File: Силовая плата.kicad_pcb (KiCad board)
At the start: 6 copper layers, 65.7 x 72.2 mm, 57 parts, among them J3 Conn_01x01, J4 Conn_01x01, J5 Conn_01x01, J6 Conn_02x04_Odd_Even, Q1 BSP89, Q2 BSP89, Q3 BSP89, Q4 BSP89, Q5 BSP89, Q6 BSP89, U1 LMV7239M5, U6 AD8210

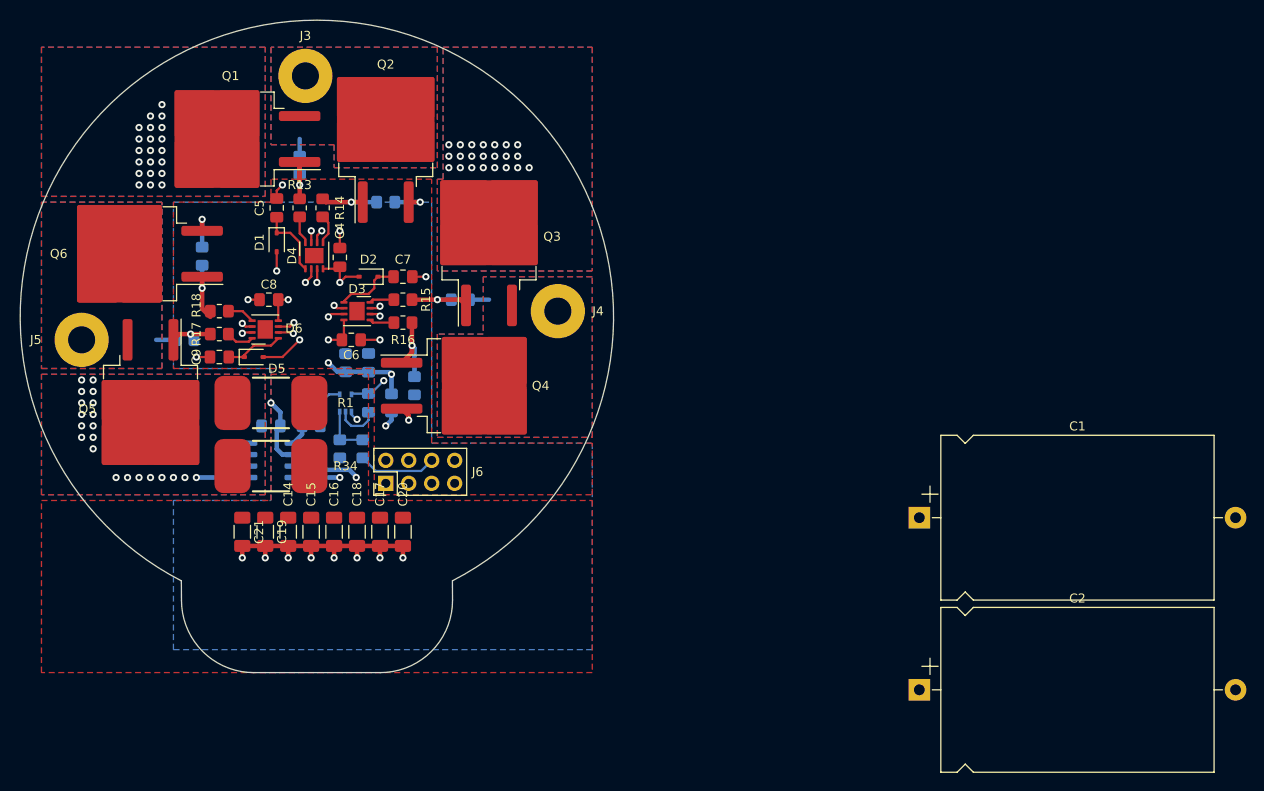
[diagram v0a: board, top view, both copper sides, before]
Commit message: Стартовая версия
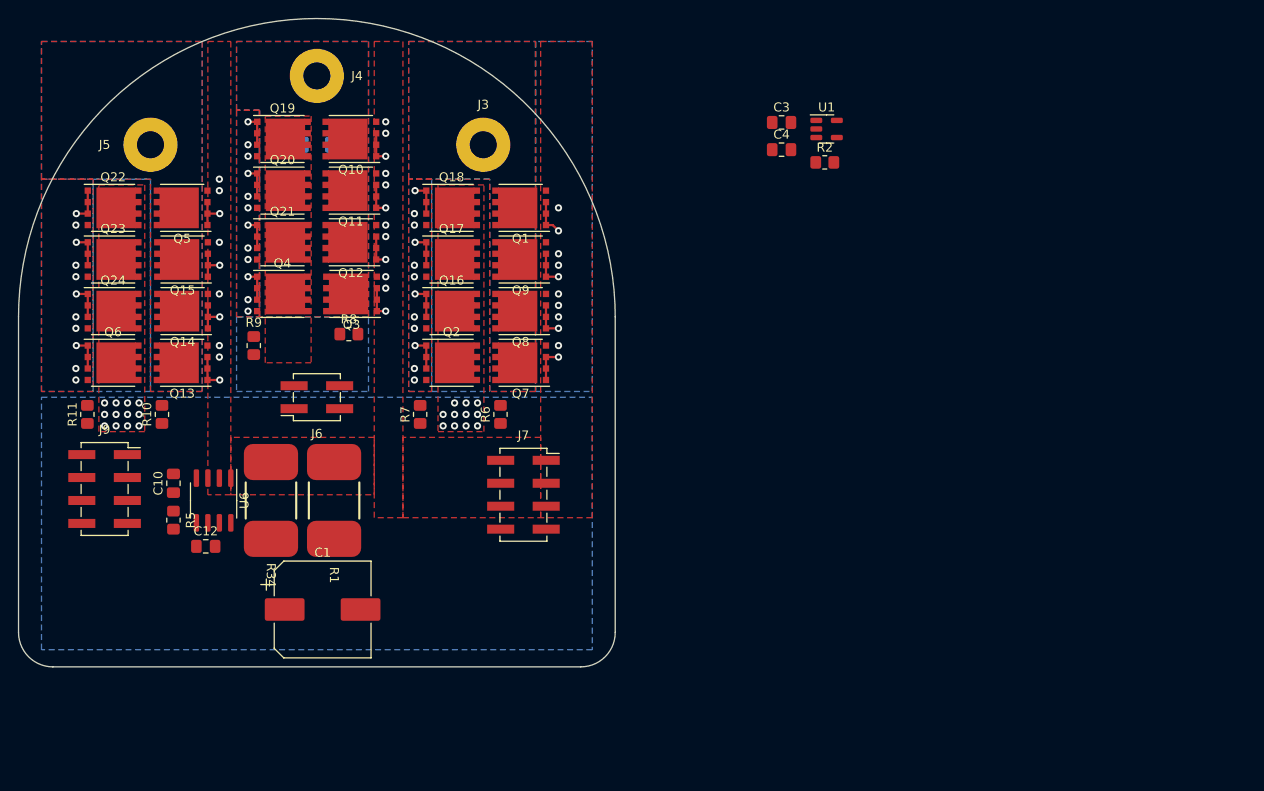
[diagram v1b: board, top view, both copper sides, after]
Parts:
- removed C11: 56p, Capacitor_SMD:C_0805_2012Metric_Pad1.18x1.45mm_HandSolder
- removed C14, C15, C16, C17, C18, C19, C20, C21: 4.7u, Capacitor_SMD:C_1206_3216Metric_Pad1.33x1.80mm_HandSolder
- removed C2: 1400m, Capacitor_THT:CP_Axial_L30.0mm_D18.0mm_P35.00mm_Horizontal
- removed C5, C7, C9: BS, Capacitor_SMD:C_0805_2012Metric_Pad1.18x1.45mm_HandSolder
- removed C6, C8: 10u, Capacitor_SMD:C_0805_2012Metric_Pad1.18x1.45mm_HandSolder
- removed D1, D2, D5: D_Small, Diode_SMD:D_SOD-323
- removed D3, D4, D6: ADP3110A, Package_DFN_QFN:DFN-8-1EP_3x3mm_P0.65mm_EP1.7x2.05mm
- removed R13, R14, R15, R16, R17, R18: 2.7, Resistor_SMD:R_0805_2012Metric_Pad1.20x1.40mm_HandSolder
- removed R21: 10k, Resistor_SMD:R_0805_2012Metric_Pad1.20x1.40mm_HandSolder
- removed R3, R4: 120, Resistor_SMD:R_0805_2012Metric_Pad1.20x1.40mm_HandSolder
- added J7: A_CTRL, Connector_PinSocket_2.54mm:PinSocket_2x04_P2.54mm_Vertical_SMD, F.Cu at (106.0, 114.3)
- added J9: C_CTRL, Connector_PinSocket_2.54mm:PinSocket_2x04_P2.54mm_Vertical_SMD, F.Cu at (59.7, 113.7)
- added Q10: BSP89, Package_SON:VSONP-8-1EP_5x6_P1.27mm, F.Cu at (87.0, 74.9)
- added Q11: BSP89, Package_SON:VSONP-8-1EP_5x6_P1.27mm, F.Cu at (87.0, 80.6)
- added Q12: BSP89, Package_SON:VSONP-8-1EP_5x6_P1.27mm, F.Cu at (87.0, 86.4)
- added Q13: BSP89, Package_SON:VSONP-8-1EP_5x6_P1.27mm, F.Cu at (68.3, 99.7)
- added Q14: BSP89, Package_SON:VSONP-8-1EP_5x6_P1.27mm, F.Cu at (68.3, 94.0)
- added Q15: BSP89, Package_SON:VSONP-8-1EP_5x6_P1.27mm, F.Cu at (68.3, 88.3)
- added Q16: BSP89, Package_SON:VSONP-8-1EP_5x6_P1.27mm, F.Cu at (98.1, 94.0)
- added Q17: BSP89, Package_SON:VSONP-8-1EP_5x6_P1.27mm, F.Cu at (98.1, 88.3)
- added Q18: BSP89, Package_SON:VSONP-8-1EP_5x6_P1.27mm, F.Cu at (98.1, 82.5)
- added Q19: BSP89, Package_SON:VSONP-8-1EP_5x6_P1.27mm, F.Cu at (79.4, 74.9)
- added Q20: BSP89, Package_SON:VSONP-8-1EP_5x6_P1.27mm, F.Cu at (79.4, 80.6)
- added Q21: BSP89, Package_SON:VSONP-8-1EP_5x6_P1.27mm, F.Cu at (79.4, 86.4)
- added Q22: BSP89, Package_SON:VSONP-8-1EP_5x6_P1.27mm, F.Cu at (60.6, 82.5)
- added Q23: BSP89, Package_SON:VSONP-8-1EP_5x6_P1.27mm, F.Cu at (60.6, 88.3)
- added Q24: BSP89, Package_SON:VSONP-8-1EP_5x6_P1.27mm, F.Cu at (60.6, 94.0)
- added Q7: BSP89, Package_SON:VSONP-8-1EP_5x6_P1.27mm, F.Cu at (105.7, 99.7)
- added Q8: BSP89, Package_SON:VSONP-8-1EP_5x6_P1.27mm, F.Cu at (105.7, 94.0)
- added Q9: BSP89, Package_SON:VSONP-8-1EP_5x6_P1.27mm, F.Cu at (105.7, 88.3)
- added TH1: 10k, Resistor_SMD:R_1206_3216Metric_Pad1.30x1.75mm_HandSolder, B.Cu at (83.2, 75.6)
- C1: footprint Capacitor_THT:CP_Axial_L30.0mm_D18.0mm_P35.00mm_Horizontal -> Capacitor_SMD:CP_Elec_10x12.5
- C10, C12, R10, R11, R5, R6, R7, R8, R9, U6: moved to F.Cu
- C3: value 0.1u -> 100n; moved to F.Cu
- C4: value 10u -> 100n
- J6: value Conn_02x04_Odd_Even -> B_CTRL; footprint Connector_PinHeader_2.54mm:PinHeader_2x04_P2.54mm_Vertical -> Connector_PinSocket_2.54mm:PinSocket_2x02_P2.54mm_Vertical_SMD
- Q1, Q2, Q3, Q4, Q5, Q6: footprint Package_TO_SOT_SMD:TO-263-2 -> Package_SON:VSONP-8-1EP_5x6_P1.27mm
- R2: value 120 -> 10k; moved to F.Cu
- U1: value LMV7239M5 -> AD8603; footprint Package_TO_SOT_SMD:SOT-353_SC-70-5 -> Package_TO_SOT_SMD:TSOT-23-5; moved to F.Cu
- moved C1 66.8 mm to (83.8, 127.0)
- moved U1 61.3 mm to (139.6, 73.8), turned to 0 degrees
- moved C3 55.3 mm to (134.6, 73.1), turned to 0 degrees
- moved R2 54.8 mm to (139.4, 77.5), turned to 0 degrees
- moved C4 50.3 mm to (134.6, 76.1), turned to 0 degrees
- moved J4 37.3 mm to (83.2, 55.8)
- moved R6 35.4 mm to (103.5, 105.4), turned to 90 degrees
- moved Q1 33.0 mm to (105.7, 82.5)
- moved Q2 26.5 mm to (98.1, 99.7), turned to 0 degrees
- moved R7 23.8 mm to (94.6, 105.4), turned to 90 degrees
- moved Q4 23.2 mm to (79.4, 92.1)
- moved J5 22.9 mm to (64.8, 63.4)
- moved Q5 22.5 mm to (68.3, 82.5), turned to 180 degrees
- moved R11 21.6 mm to (57.8, 105.4), turned to 90 degrees
- moved J3 21.1 mm to (101.6, 63.4)
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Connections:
- C12 pad 1: Net-(U1--) -> DC_Measure
- C3 pad 1: +5V -> Net-(U1-+)
- C4 pad 1: GND -> +5V
- C4 pad 2: +12V -> GND
- J6 pad 1: IN_A -> G3
- J6 pad 2: GND -> G4
- J6 pad 3: IN_B -> B
- J6 pad 4: +12V -> GND
- R2 pad 1: Net-(R2-Pad1) -> +5V
- R2 pad 2: Enable -> Net-(U1-+)
- R5 pad 1: Net-(U1--) -> DC_Measure
- R5 pad 2: DC_Measure -> Net-(U6-OUT)
- U1 pad 1: Net-(R2-Pad1) -> Temp_out
- U1 pad 4: Net-(U1--) -> Temp_out
- U6 pad 5: DC_Measure -> Net-(U6-OUT)
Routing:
- net GND: track 52.5 -> 0.00 mm, vias 17 -> 23
- net +5V: track 45.9 -> 0.00 mm, vias 2 -> 0
- net +12V: track 43.1 -> 0.00 mm, vias 5 -> 0
- net DC_Measure: track 32.3 -> 0.00 mm, vias 1 -> 0
- net IN_C: track 31.8 -> 0.00 mm, vias 1 -> 0
- net IN_B: track 30.0 -> 0.00 mm, vias 1 -> 0
- net Enable: track 29.9 -> 0.00 mm, vias 5 -> 0
- net IN_A: track 28.7 -> 0.00 mm, vias 1 -> 0
- net B: track 18.6 -> 0.00 mm, vias 2 -> 8
- net A: track 16.1 -> 0.00 mm, vias 2 -> 8
- net C: track 15.4 -> 0.00 mm, vias 2 -> 7
- net G5: track 5.13 -> 15.6 mm, vias 1 -> 4
- net G1: track 7.80 -> 16.0 mm, vias 1 -> 4
- net Net-(D1-K): track 7.89 -> 0.00 mm
- net G6: track 7.36 -> 15.2 mm, vias 1 -> 4
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- added copper zone on In2.Cu, net G1
- added copper zone on In2.Cu, net G2
- added copper zone on In2.Cu, net G3
- added copper zone on In2.Cu, net G4
- added copper zone on In2.Cu, net G5
- added copper zone on In2.Cu, net G6
- removed copper zone on In2.Cu, net +12V
- removed copper zone on In1.Cu, net A
- removed copper zone on In2.Cu, net A
- removed copper zone on In3.Cu, net A
- removed copper zone on In4.Cu, net A
- removed copper zone on In1.Cu, net B
- removed copper zone on In2.Cu, net B
- removed copper zone on In3.Cu, net B
- removed copper zone on In4.Cu, net B
- removed copper zone on In1.Cu, net C
- removed copper zone on In2.Cu, net C
- removed copper zone on In3.Cu, net C
- removed copper zone on In4.Cu, net C
- removed copper zone on In1.Cu, net Enable
- removed copper zone on F.Cu, net Shunt_1
- removed copper zone on B.Cu, net Shunt_2
- removed copper zone on In1.Cu, net Shunt_2
- removed copper zone on In4.Cu, net Shunt_2
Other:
- board size 65.7 x 72.2 mm -> 66 x 71.8 mm
